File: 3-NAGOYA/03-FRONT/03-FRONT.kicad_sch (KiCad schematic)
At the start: 16 parts, among them J6 OpenMV Conn

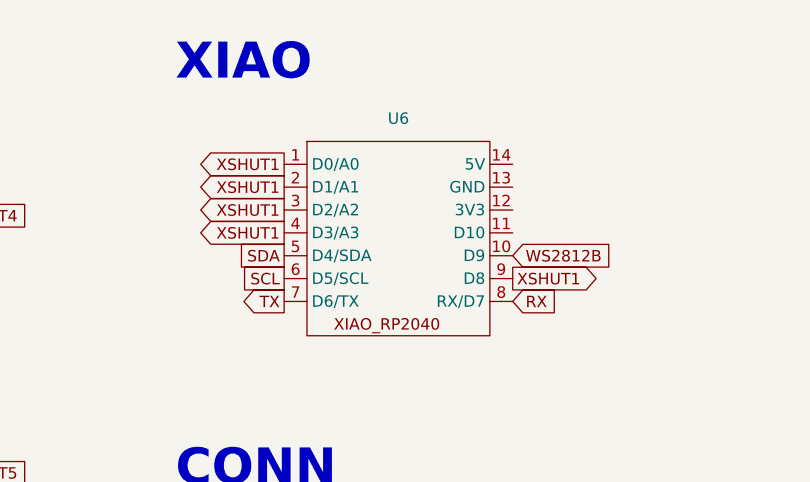
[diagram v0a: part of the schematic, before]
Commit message: 06-UI完成
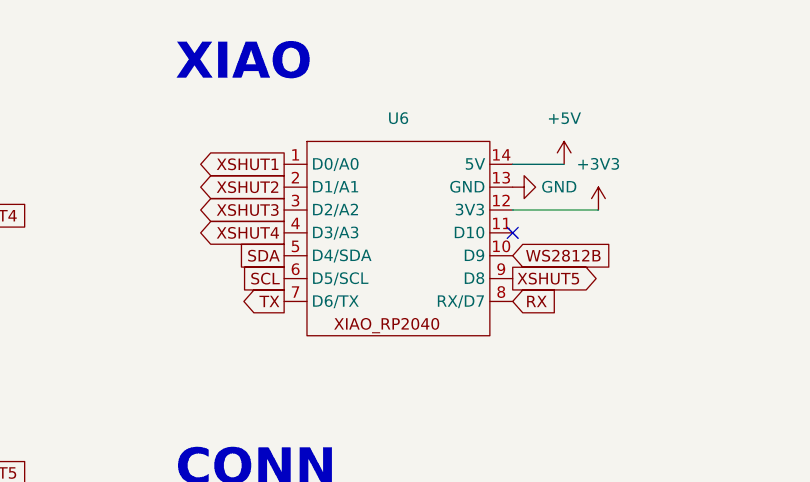
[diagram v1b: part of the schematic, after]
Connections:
- net +3V3: now also U6.12 (3V3)
- net +5V: now also U6.14 (5V)
- net GND: now also U6.13 (GND)
- net XSHUT1: no longer U6.2 (D1/A1), U6.3 (D2/A2), U6.4 (D3/A3), U6.9 (D8)
- net XSHUT2: now also U6.2 (D1/A1)
- net XSHUT3: now also U6.3 (D2/A2)
- net XSHUT4: now also U6.4 (D3/A3)
- net XSHUT5: now also U6.9 (D8)
- no-connect marks 6 -> 7
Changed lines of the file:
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@@
   (no_connect (at 50.8 48.26))
   (no_connect (at 50.8 75.565))
+  (no_connect (at 159.385 46.99))
   (no_connect (at 95.885 48.26))
   (no_connect (at 50.8 102.87))
@@
     (stroke (width 0) (type default))
   )
+  (wire (pts (xy 168.91 44.45) (xy 159.385 44.45))
+    (stroke (width 0) (type default))
+  )
   (wire (pts (xy 49.53 156.21) (xy 71.12 156.21))
     (stroke (width 0) (type default))
@@
   )
   (wire (pts (xy 86.995 99.695) (xy 83.82 99.695))
+    (stroke (width 0) (type default))
+  )
+  (wire (pts (xy 165.1 39.37) (xy 159.385 39.37))
     (stroke (width 0) (type default))
   )
@@
     )
   )
-  (global_label "XSHUT1" (shape output) (at 133.985 41.91 180) (fields_autoplaced)
+  (global_label "XSHUT2" (shape output) (at 133.985 41.91 180) (fields_autoplaced)
     (effects (font (size 1.27 1.27)) (justify right))
     (property "Intersheetrefs" "${INTERSHEET_REFS}" (at 123.7427 41.91 0)
@@
     )
   )
-  (global_label "XSHUT1" (shape output) (at 159.385 52.07 0) (fields_autoplaced)
+  (global_label "XSHUT5" (shape output) (at 159.385 52.07 0) (fields_autoplaced)
     (effects (font (size 1.27 1.27)) (justify left))
     (property "Intersheetrefs" "${INTERSHEET_REFS}" (at 169.6273 52.07 0)
@@
     )
   )
-  (global_label "XSHUT1" (shape output) (at 133.985 44.45 180) (fields_autoplaced)
+  (global_label "XSHUT3" (shape output) (at 133.985 44.45 180) (fields_autoplaced)
     (effects (font (size 1.27 1.27)) (justify right))
     (property "Intersheetrefs" "${INTERSHEET_REFS}" (at 123.7427 44.45 0)
@@
     )
   )
-  (global_label "XSHUT1" (shape output) (at 133.985 46.99 180) (fields_autoplaced)
+  (global_label "XSHUT4" (shape output) (at 133.985 46.99 180) (fields_autoplaced)
     (effects (font (size 1.27 1.27)) (justify right))
     (property "Intersheetrefs" "${INTERSHEET_REFS}" (at 123.7427 46.99 0)
@@
         (path "/e118ed56-ce79-44d8-8eff-a935fd9f7b40"
           (reference "D2") (unit 1)
+        )
+      )
+    )
+  )
+  (symbol (lib_id "power:+3V3") (at 168.91 44.45 0) (unit 1)
+    (in_bom yes) (on_board yes) (dnp no) (fields_autoplaced)
+    (property "Reference" "#PWR018" (at 168.91 48.26 0)
+      (effects (font (size 1.27 1.27)) hide)
+    )
+    (property "Value" "+3V3" (at 168.91 39.37 0)
+      (effects (font (size 1.27 1.27)))
+    )
+    (property "Footprint" "" (at 168.91 44.45 0)
+      (effects (font (size 1.27 1.27)) hide)
+    )
+    (property "Datasheet" "" (at 168.91 44.45 0)
+      (effects (font (size 1.27 1.27)) hide)
+    )
+    (pin "1")
+    (instances
+      (project "03-FRONT"
+        (path "/e118ed56-ce79-44d8-8eff-a935fd9f7b40"
+          (reference "#PWR018") (unit 1)
+        )
+      )
+    )
+  )
+  (symbol (lib_id "power:GND") (at 159.385 41.91 90) (unit 1)
+    (in_bom yes) (on_board yes) (dnp no) (fields_autoplaced)
+    (property "Reference" "#PWR019" (at 165.735 41.91 0)
+      (effects (font (size 1.27 1.27)) hide)
+    )
+    (property "Value" "GND" (at 162.56 41.91 90)
+      (effects (font (size 1.27 1.27)) (justify right))
+    )
+    (property "Footprint" "" (at 159.385 41.91 0)
+      (effects (font (size 1.27 1.27)) hide)
+    )
+    (property "Datasheet" "" (at 159.385 41.91 0)
+      (effects (font (size 1.27 1.27)) hide)
+    )
+    (pin "1")
+    (instances
+      (project "03-FRONT"
+        (path "/e118ed56-ce79-44d8-8eff-a935fd9f7b40"
+          (reference "#PWR019") (unit 1)
         )
       )
@@
         )
       )
+    )
+  )
+  (symbol (lib_id "power:+5V") (at 165.1 39.37 0) (unit 1)
+    (in_bom yes) (on_board yes) (dnp no) (fields_autoplaced)
+    (property "Reference" "#PWR017" (at 165.1 43.18 0)
+      (effects (font (size 1.27 1.27)) hide)
+    )
+    (property "Value" "+5V" (at 165.1 34.29 0)
+      (effects (font (size 1.27 1.27)))
+    )
+    (property "Footprint" "" (at 165.1 39.37 0)
+      (effects (font (size 1.27 1.27)) hide)
+    )
+    (property "Datasheet" "" (at 165.1 39.37 0)
+      (effects (font (size 1.27 1.27)) hide)
+    )
+    (pin "1")
+    (instances
+      (project "03-FRONT"
+        (path "/e118ed56-ce79-44d8-8eff-a935fd9f7b40"
+          (reference "#PWR017") (unit 1)
+        )
+      )
